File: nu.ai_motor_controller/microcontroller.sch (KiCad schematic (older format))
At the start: 35 parts, among them J10 Conn_02x05_Odd_Even, J11 DX4R105JJCR1800, J9 Conn_02x12_Odd_Even, SW1 TACTILE_SWITCH, U9 ATmega32U4-AU, Y1 7M-16.000MAAE-T

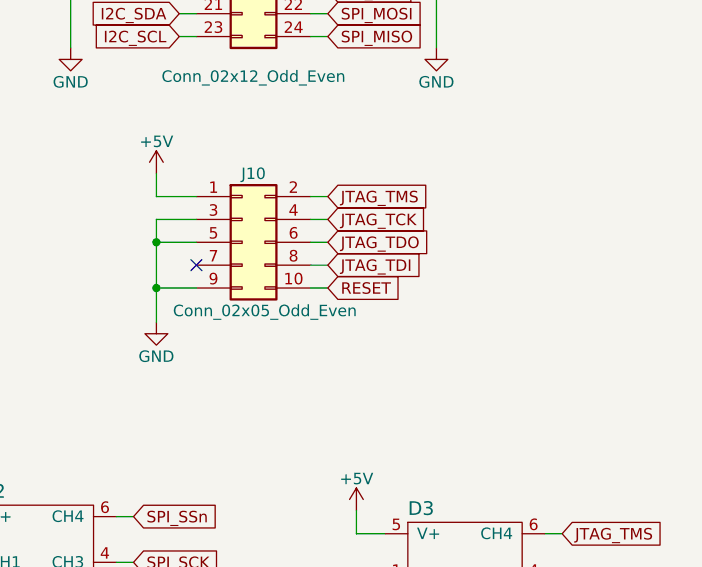
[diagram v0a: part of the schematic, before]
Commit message: automated commit
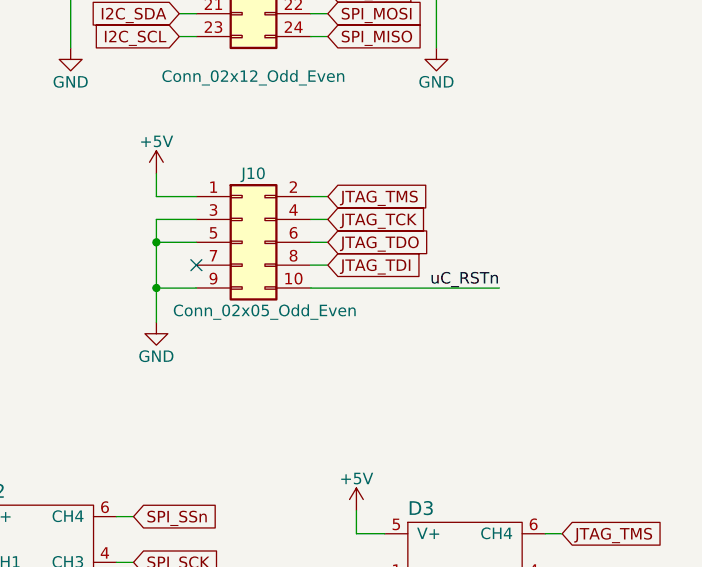
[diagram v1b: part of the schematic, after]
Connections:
- net RESET is gone; now on net uC_RSTn: J10.10 (Pin_10)
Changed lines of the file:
@@
 	1    0    0    -1
 $EndComp
-Text GLabel 9525 3175 2    50   Input ~ 0
-RESET
-Wire Wire Line
-	9525 3175 9450 3175
+Wire Wire Line
+	10275 3175 9450 3175
 Wire Wire Line
 	4450 2150 4450 2450
@@
 Wire Wire Line
 	1150 1325 1550 1325
+Text Label 10275 3175 2    50   ~ 0
+uC_RSTn
 $EndSCHEMATC
